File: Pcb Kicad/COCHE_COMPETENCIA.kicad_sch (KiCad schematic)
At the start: 35 parts, among them J1 BAT, J2 SWITCH, J4 M1, J5 M2, J6 SENSORES, Q1 2N3904, SW1 SW_Push, SW2 SW_Push, U2 ESP32-DEVKIT-V1, U3 DRV8833, U4 DRV8833, U5 AMS1117

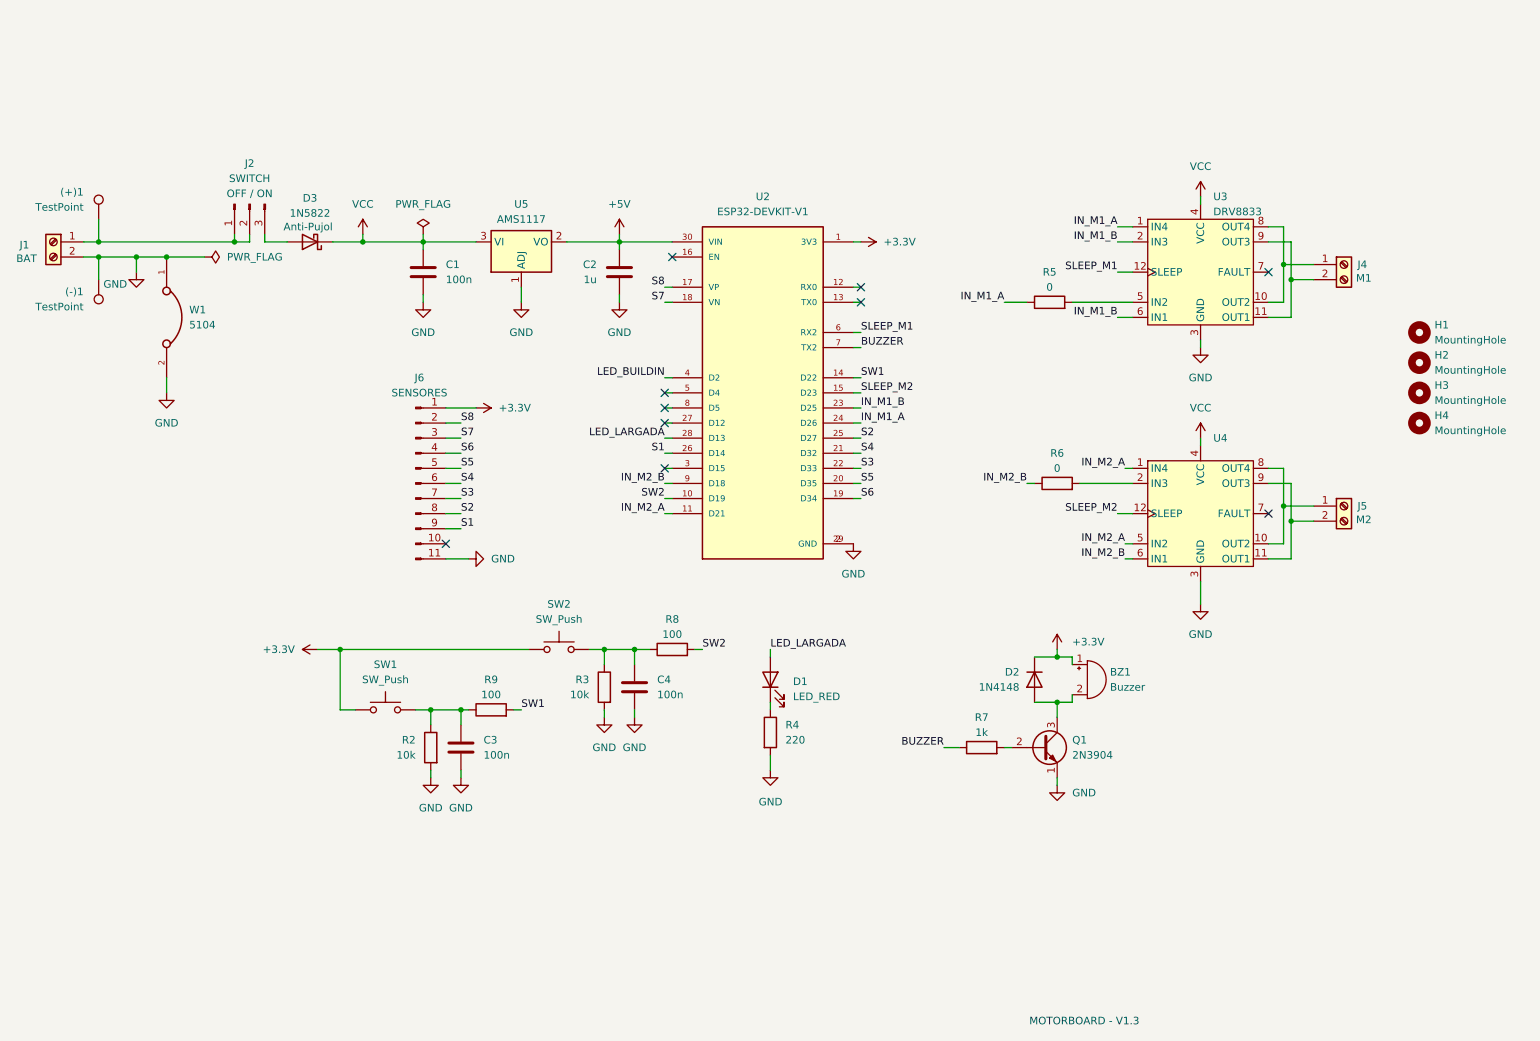
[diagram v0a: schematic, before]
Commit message: V2.0 - Nueva version Seguidor De Linea
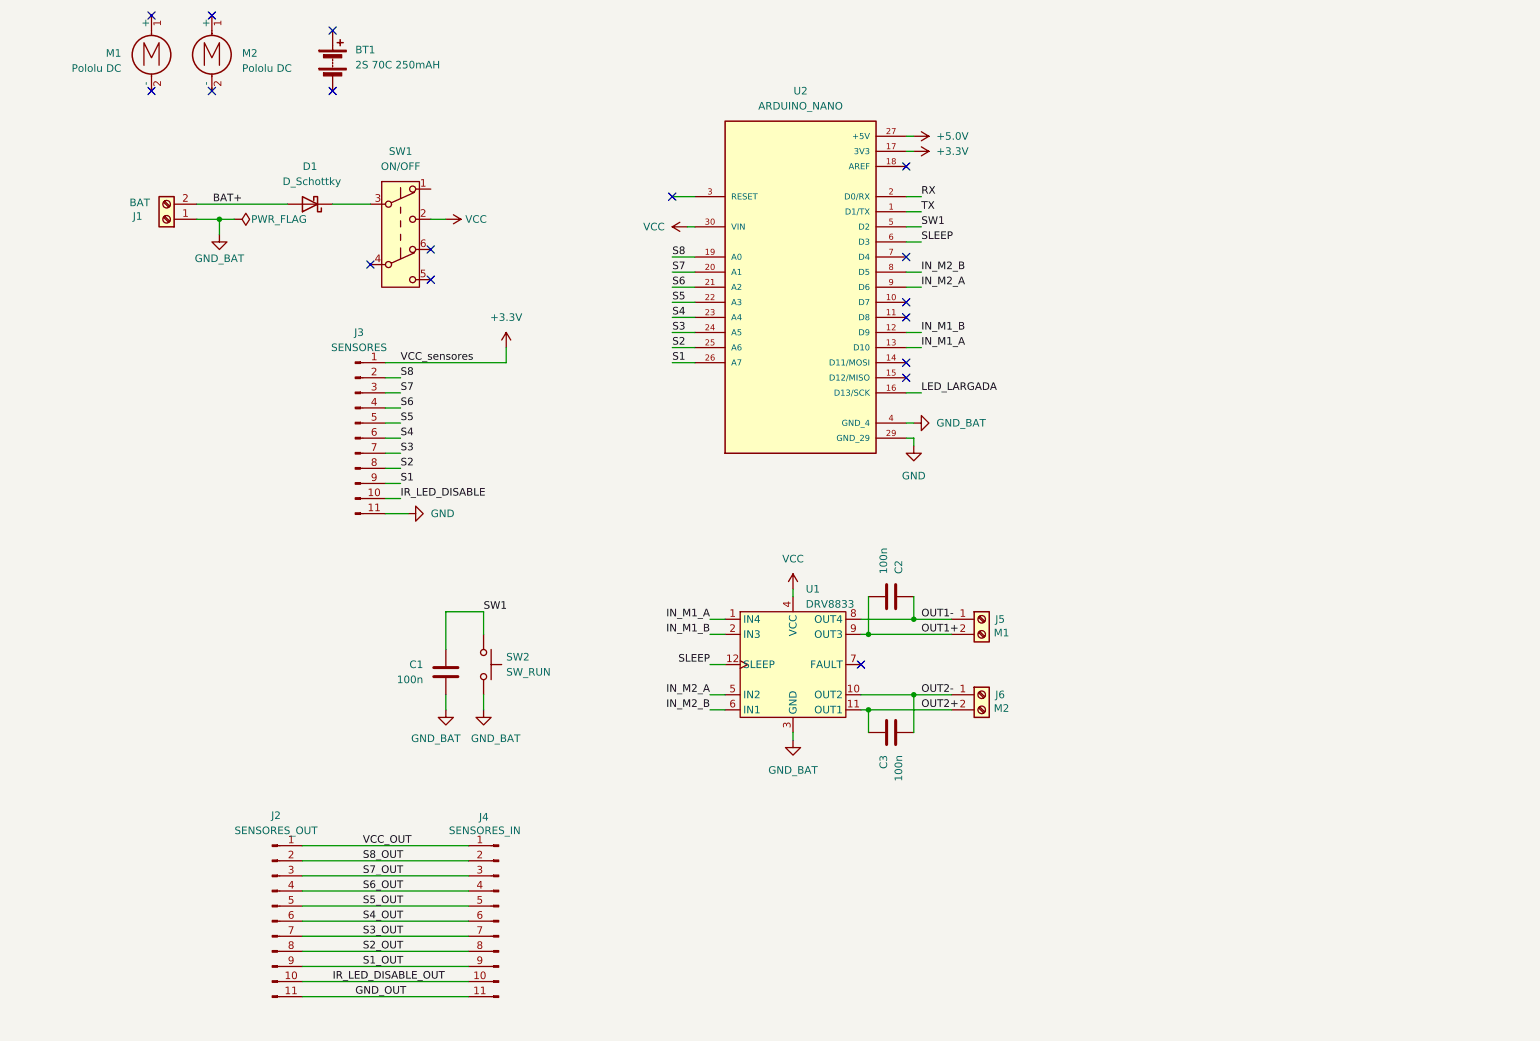
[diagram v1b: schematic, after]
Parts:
- removed (+)1, (-)1: TestPoint, Connector_PinHeader_2.54mm:PinHeader_1x01_P2.54mm_Vertical, symbol Connector:TestPoint
- removed BZ1: Buzzer, Buzzer_Beeper:MagneticBuzzer_ProSignal_ABI-009-RC, symbol Device:Buzzer
- removed C1, C4: 100n, Capacitor_SMD:C_1206_3216Metric_Pad1.33x1.80mm_HandSolder, symbol Device:C
- removed D1: LED_RED, LED_THT:LED_D5.0mm, symbol Device:LED
- removed D2: 1N4148, Diode_THT:D_DO-35_SOD27_P7.62mm_Horizontal, symbol Diode:1N4148
- removed D3: 1N5822, Diode_THT:D_DO-201AD_P12.70mm_Horizontal, symbol Diode:1N5822
- removed H1, H2, H3, H4: MountingHole, MountingHole:MountingHole_3mm, symbol Mechanical:MountingHole
- removed J2: SWITCH, Connector_PinHeader_2.54mm:PinHeader_1x03_P2.54mm_Vertical, symbol Connector:Conn_01x03_Pin
- removed Q1: 2N3904, Package_TO_SOT_THT:TO-92_Inline_Wide, symbol Transistor_BJT:2N3904
- removed R2, R3: 10k, Resistor_SMD:R_1206_3216Metric_Pad1.30x1.75mm_HandSolder, symbol Device:R
- removed R4: 220, Resistor_SMD:R_1206_3216Metric_Pad1.30x1.75mm_HandSolder, symbol Device:R
- removed R5, R6: 0, Resistor_SMD:R_1206_3216Metric_Pad1.30x1.75mm_HandSolder, symbol Device:R
- removed R7: 1k, Resistor_SMD:R_1206_3216Metric_Pad1.30x1.75mm_HandSolder, symbol Device:R
- removed R8, R9: 100, Resistor_SMD:R_1206_3216Metric_Pad1.30x1.75mm_HandSolder, symbol Device:R
- removed SW2: SW_Push, Button_Switch_THT:SW_PUSH_6mm_H5mm, symbol Switch:SW_Push
- removed U2: ESP32-DEVKIT-V1, ESP32-DEVKIT-V1:MODULE_ESP32_DEVKIT_V1, symbol ESP32-DEVKIT-V1:ESP32-DEVKIT-V1
- removed U4: DRV8833, DRV8833:DRV8833, symbol DRV8833_Module:DRV8833_Module
- removed U5: AMS1117, Package_TO_SOT_SMD:SOT-223-3_TabPin2, symbol Regulator_Linear:AMS1117
- removed W1: 5104, JUMPLER 5104:KEYSTONE_5104, symbol 5104:5104
- added BT1: 2S 70C 250mAH, Bateria_9S:Bateria_Lado, symbol Device:Battery
- added C3: 100n, Capacitor_SMD:C_1206_3216Metric_Pad1.33x1.80mm_HandSolder, symbol Device:C
- added D1: D_Schottky, Diode_THT:D_DO-35_SOD27_P7.62mm_Horizontal, symbol Device:D_Schottky
- added J2: SENSORES_OUT, Connector_PinHeader_2.54mm:PinHeader_1x11_P2.54mm_Vertical, symbol Connector:Conn_01x11_Pin
- added J4: SENSORES_IN, Connector_PinHeader_2.54mm:PinHeader_1x11_P2.54mm_Vertical, symbol Connector:Conn_01x11_Pin
- added M1, M2: Pololu DC, PololuLibrary:pololu, symbol Motor:Motor_DC
- added SW1: ON/OFF, switch6P:SWITCH_6PINS, symbol Switch:SW_Push_DPDT
- added U2: ARDUINO_NANO, Arduino NANO:MODULE_ARDUINO_NANO, symbol ARDUINO_NANO:ARDUINO_NANO
- C2: value 1u -> 100n
- J1: footprint TerminalBlock_Phoenix:TerminalBlock_Phoenix_MKDS-1,5-2_1x02_P5.00mm_Horizontal -> AMASS_XT30UPB-M_1x02_P5.0mm_Vertical
- J5: renamed from J4; footprint TerminalBlock_Phoenix:TerminalBlock_Phoenix_MKDS-1,5-2_1x02_P5.00mm_Horizontal -> Connector_PinHeader_2.54mm:PinHeader_1x02_P2.54mm_Vertical
- J6: renamed from J5; footprint TerminalBlock_Phoenix:TerminalBlock_Phoenix_MKDS-1,5-2_1x02_P5.00mm_Horizontal -> Connector_PinHeader_2.54mm:PinHeader_1x02_P2.54mm_Vertical
- SW2: renamed from SW1; value SW_Push -> SW_RUN
- renumbered C3 to C1, J6 to J3, U3 to U1
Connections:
- net +5V is gone; now on net OUT1-: C2.1
- net +3.3V: now also U2.17 (3V3); no longer SW2.1
- net GND: now also U2.29 (GND_29); no longer C1.2, C2.2, J1.2 (Pin_2), U1.3 (GND)
- net IN_M1_A: now also U2.13 (D10)
- net IN_M1_B: now also U2.12 (D9); no longer U1.6 (IN1)
- net IN_M2_A: now also U1.5 (IN2), U2.9 (D6)
- net IN_M2_B: now also U1.6 (IN1), U2.8 (D5)
- net LED_LARGADA: now also U2.16 (D13/SCK)
- net S1: now also U2.26 (A7)
- net S2: now also U2.25 (A6)
- net S3: now also U2.24 (A5)
- net S4: now also U2.23 (A4)
- net S5: now also U2.22 (A3)
- net S6: now also U2.21 (A2)
- net S7: now also U2.20 (A1)
- net S8: now also U2.19 (A0)
- net SW1: now also C1.1, SW2.1, U2.5 (D2)
- net VCC: now also SW1.2 (C), U2.30 (VIN)
- net GND_BAT: now reaches SW2.2
- net GND_BAT: now also C1.2, J1.1 (Pin_1), U1.3 (GND), U2.4 (GND_4); no longer C1.1
- net OUT1-: now reaches J5.1 (Pin_1), U1.8 (OUT4)
- net OUT1-: no longer U1.10 (OUT2)
- net OUT1+: now reaches J5.2 (Pin_2), U1.9 (OUT3)
- net OUT1+: now also C2.2; no longer U1.11 (OUT1)
- net IR_LED_DISABLE: now reaches J3.10 (Pin_10)
- net OUT2-: now reaches J6.1 (Pin_1)
- net OUT2-: now also U1.10 (OUT2), C3.2
- net OUT2+: now reaches J6.2 (Pin_2)
- net OUT2+: now also U1.11 (OUT1), C3.1
- net SLEEP_M1 renamed SLEEP
- net SLEEP: now also U2.6 (D3)
- new net: D1.1 (K), SW1.3 (B)
- new net: U2.28 (RESET), U2.3 (RESET)
- new net +5.0V: U2.27 (+5V)
- new net BAT+: D1.2 (A), J1.2 (Pin_2)
- new net GND_OUT: J2.11 (Pin_11), J4.11 (Pin_11)
- new net IR_LED_DISABLE_OUT: J2.10 (Pin_10), J4.10 (Pin_10)
- new net RX: U2.2 (D0/RX)
- new net S1_OUT: J2.9 (Pin_9), J4.9 (Pin_9)
- new net S2_OUT: J2.8 (Pin_8), J4.8 (Pin_8)
- new net S3_OUT: J2.7 (Pin_7), J4.7 (Pin_7)
- new net S4_OUT: J2.6 (Pin_6), J4.6 (Pin_6)
- new net S5_OUT: J2.5 (Pin_5), J4.5 (Pin_5)
- new net S6_OUT: J2.4 (Pin_4), J4.4 (Pin_4)
- new net S7_OUT: J2.3 (Pin_3), J4.3 (Pin_3)
- new net S8_OUT: J2.2 (Pin_2), J4.2 (Pin_2)
- new net TX: U2.1 (D1/TX)
- new net VCC_OUT: J2.1 (Pin_1), J4.1 (Pin_1)
- no-connect marks 10 -> 17
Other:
- note removed: "MOTORBOARD - V1.3"
- company: (none) -> FIE
- title: (none) -> MotorBoard
- moved on the sheet: C1, J1, J3, J5, J6, SW2, U1
